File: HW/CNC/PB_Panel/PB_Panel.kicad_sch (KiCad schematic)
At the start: 19 parts, among them J1 1x11 2.54mm female 90deg, SW1 RED, SW10 RED, SW11 BLUE, SW12 BLUE, SW13 YELLOW, SW14 YELLOW, SW15 GRAY, SW16 GRAY, SW17 BLACK, SW18 BLACK, SW2 RED, SW3 GREEN, SW4 GREEN, SW5 BLUE, SW6 BLUE, SW7 RED, SW8 RED, SW9 GREEN

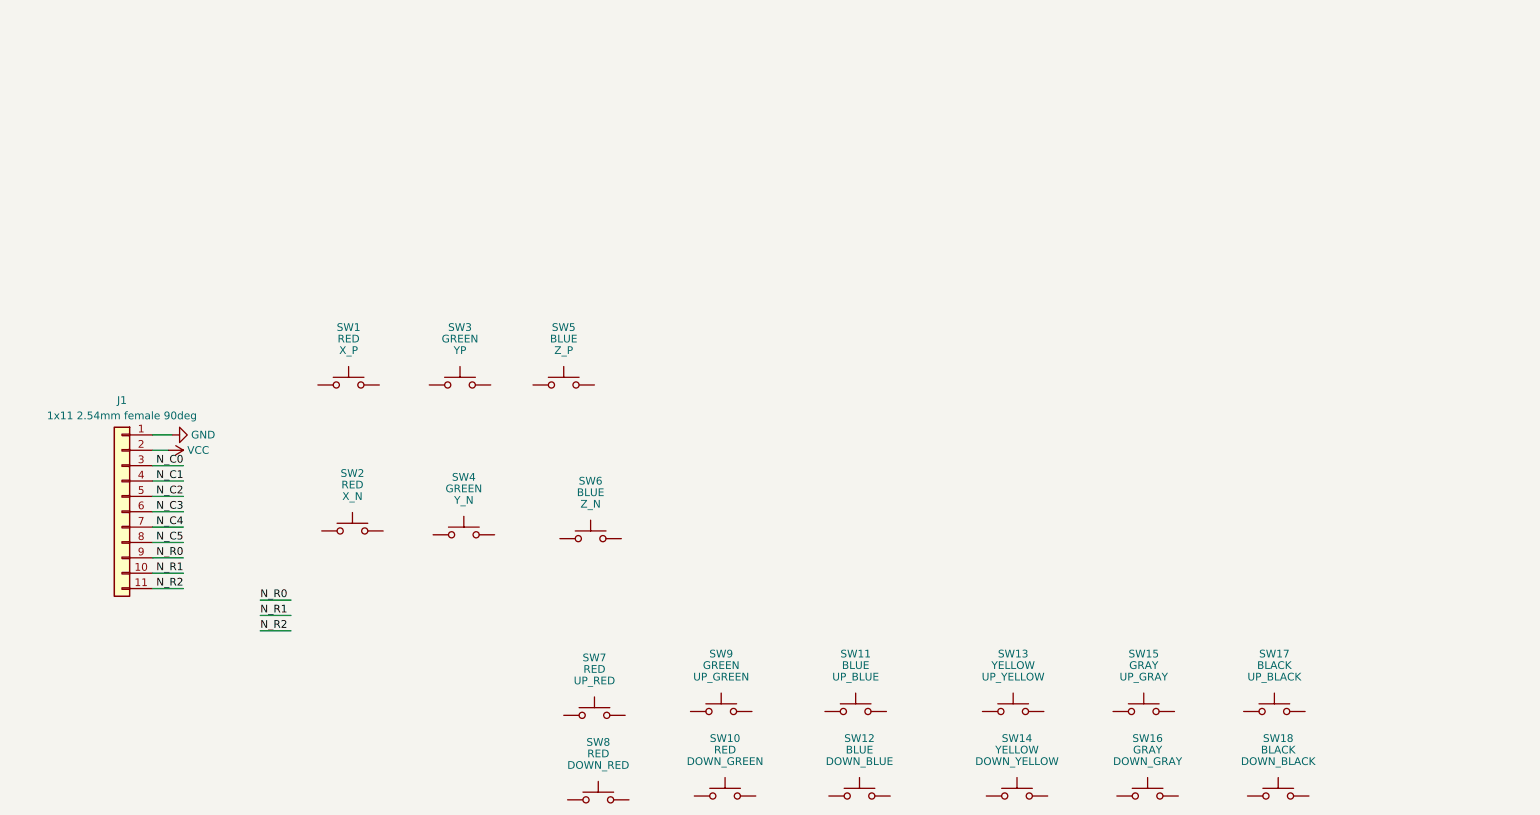
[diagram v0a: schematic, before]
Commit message: Finished PCB.
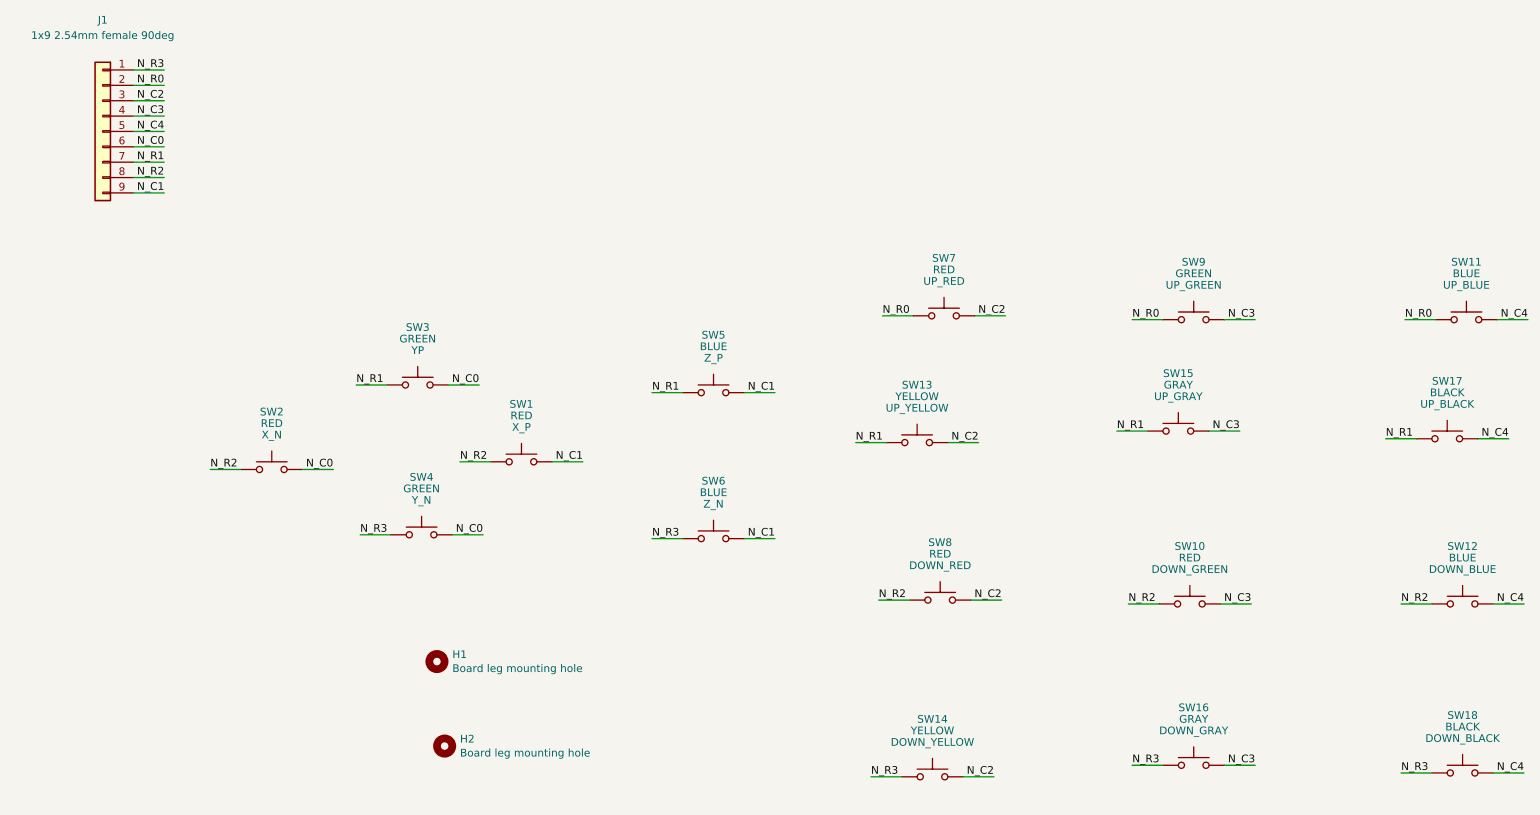
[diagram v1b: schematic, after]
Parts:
- added H1, H2: Board leg mounting hole, MountingHole:MountingHole_3.2mm_M3, symbol Mechanical:MountingHole
- J1: value 1x11 2.54mm female 90deg -> 1x9 2.54mm female 90deg; footprint Connector_PinSocket_2.54mm:PinSocket_1x11_P2.54mm_Horizontal -> Connector_PinSocket_2.54mm:PinSocket_1x09_P2.54mm_Horizontal; symbol Connector_Generic:Conn_01x11 -> Connector_Generic:Conn_01x09
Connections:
- net GND is gone; now on net N_R3: J1.1 (Pin_1)
- net N_C5 is gone; now on net N_R2: J1.8 (Pin_8)
- net VCC is gone; now on net N_R0: J1.2 (Pin_2)
- net N_C0: now also J1.6 (Pin_6), SW2.1, SW3.1, SW4.1; no longer J1.3 (Pin_3)
- net N_C1: now also J1.9 (Pin_9), SW1.1, SW5.1, SW6.1; no longer J1.4 (Pin_4)
- net N_C2: now also J1.3 (Pin_3), SW13.1, SW14.1, SW7.1, SW8.1; no longer J1.5 (Pin_5)
- net N_C3: now also J1.4 (Pin_4), SW10.1, SW15.1, SW16.1, SW9.1; no longer J1.6 (Pin_6)
- net N_C4: now also J1.5 (Pin_5), SW11.1, SW12.1, SW17.1, SW18.1; no longer J1.7 (Pin_7)
- net N_R0: now also SW11.2, SW7.2, SW9.2; no longer J1.9 (Pin_9)
- net N_R1: now also J1.7 (Pin_7), SW13.2, SW15.2, SW17.2, SW3.2, SW5.2; no longer J1.10 (Pin_10)
- net N_R2: now also SW1.2, SW10.2, SW12.2, SW2.2, SW8.2; no longer J1.11 (Pin_11)
- net N_R3: now reaches SW4.2
- net N_R3: now also SW14.2, SW16.2, SW18.2, SW6.2
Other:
- moved on the sheet: SW1, SW10, SW11, SW12, SW13, SW14, SW15, SW16, SW17, SW18, SW2, SW3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
